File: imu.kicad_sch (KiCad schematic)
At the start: 4 parts, among them U6 MPU-6050

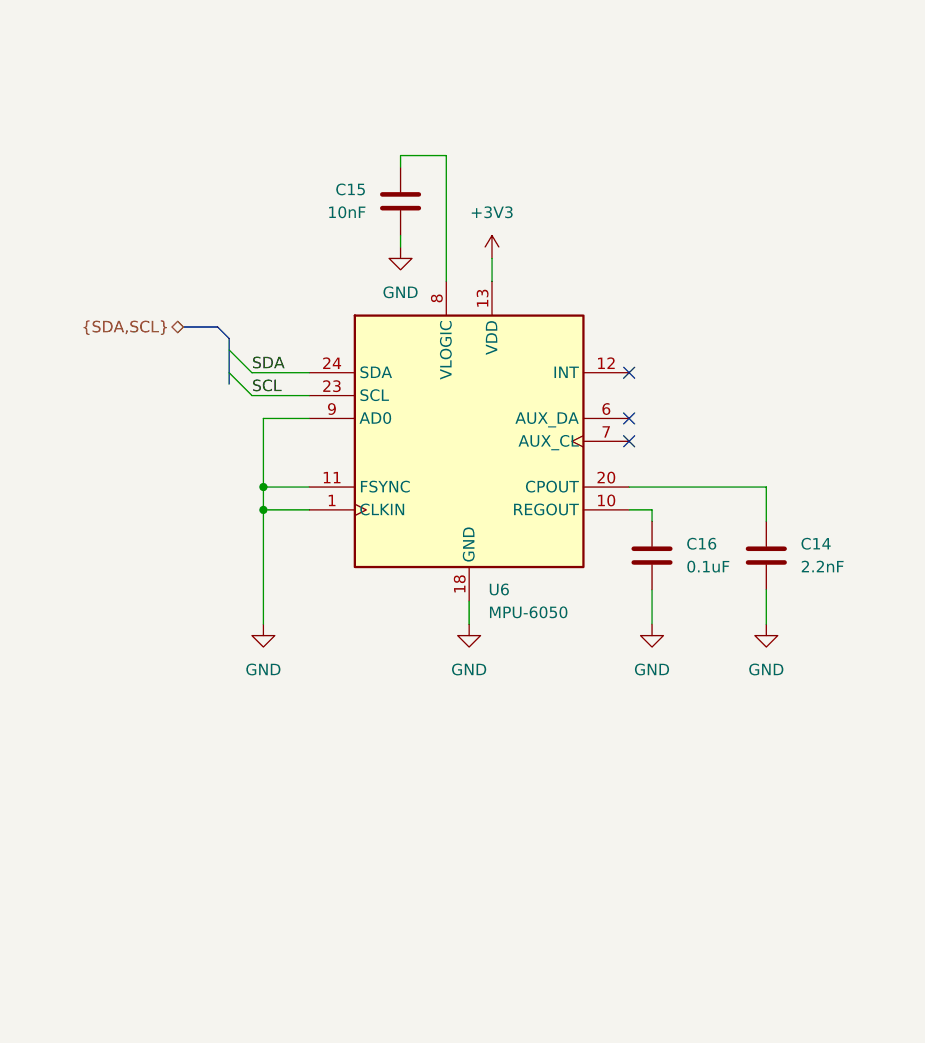
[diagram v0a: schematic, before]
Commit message: progress on routing
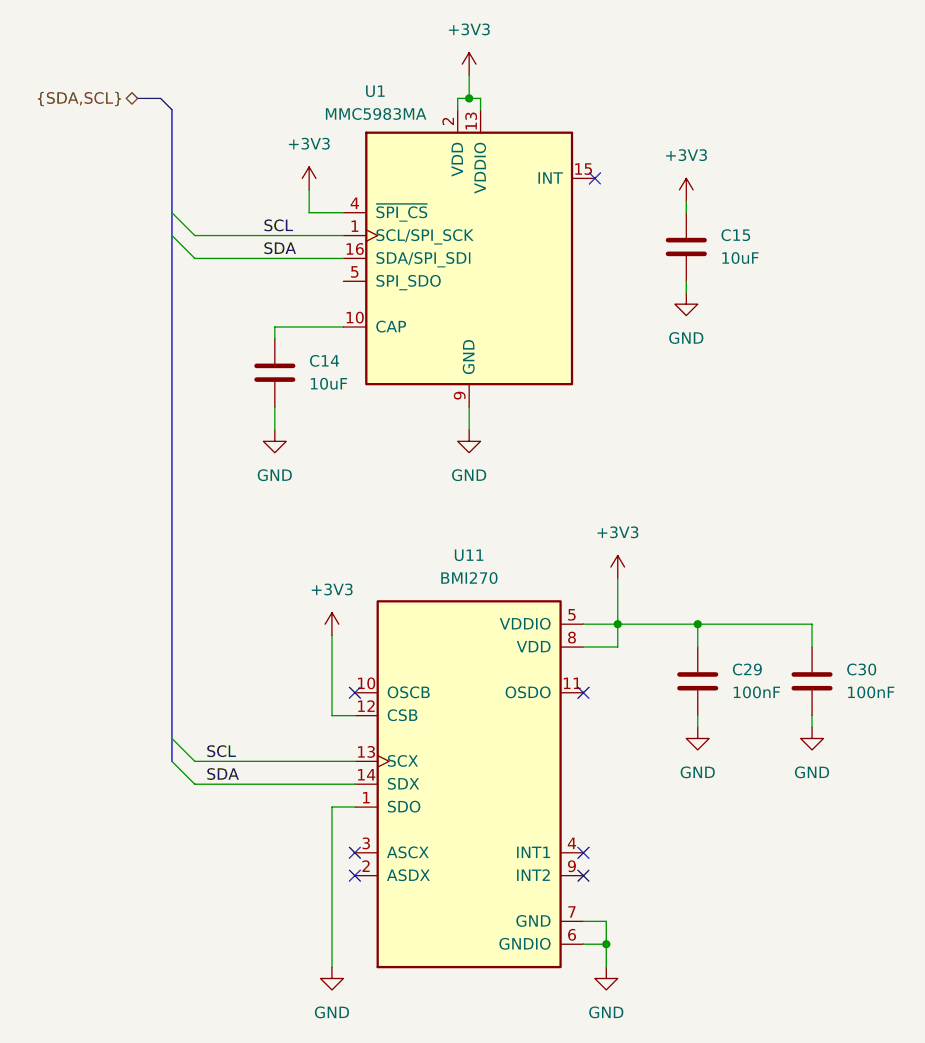
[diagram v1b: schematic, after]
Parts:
- removed C16: 0.1uF, symbol Device:C
- removed U6: MPU-6050, Sensor_Motion:InvenSense_QFN-24_4x4mm_P0.5mm, symbol Sensor_Motion:MPU-6050
- added C29, C30: 100nF, Capacitor_SMD:C_0603_1608Metric, symbol Device:C
- added U1: MMC5983MA, MMC5983MA:PQFN50P300X300X100-16N, symbol MMC5983MA:MMC5983MA
- added U11: BMI270, Package_LGA:Bosch_LGA-14_3x2.5mm_P0.5mm, symbol BMI270:BMI270
- C14: value 2.2nF -> 10uF
- C15: value 10nF -> 10uF
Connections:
- net +3V3: now also C15.1, C29.1, C30.1, U1.13 (VDDIO), U1.2 (VDD), U1.4 (~{SPI_CS}), U11.12 (CSB), U11.5 (VDDIO), U11.8 (VDD)
- net GND: now also C29.2, C30.2, U1.11 (GND), U1.9 (GND), U11.1 (SDO), U11.6 (GNDIO), U11.7 (GND)
- net SCL: now also U1.1 (SCL/SPI_SCK), U11.13 (SCX)
- net SDA: now also U1.16 (SDA/SPI_SDI), U11.14 (SDX)
- net at C14.1: now also U1.10 (CAP)
- new net: U1.12 (NC), U1.14 (NC), U1.3 (NC), U1.6 (NC), U1.7 (NC), U1.8 (NC)
- no-connect marks 3 -> 7
